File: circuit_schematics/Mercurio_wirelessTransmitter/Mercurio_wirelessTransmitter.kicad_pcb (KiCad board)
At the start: 2 copper layers, 120.6 x 52.1 mm, 61 parts, among them J1 USB_MICRO_B, J2 SIM_CARD_SLOT, J3 MAIN_ANTENNA, J4 SENSOR_IN, J5 ICSP, Q1 CSD16301Q2, Q2 CSD16301Q2, Q3 S8050, Q4 S8050, U1 ATmega8U2-MU, U2 SIM7600E-H, U3 ADS1115IDGS, U4 BQ29707DSET, U5 MT3608, Y1 16MHz

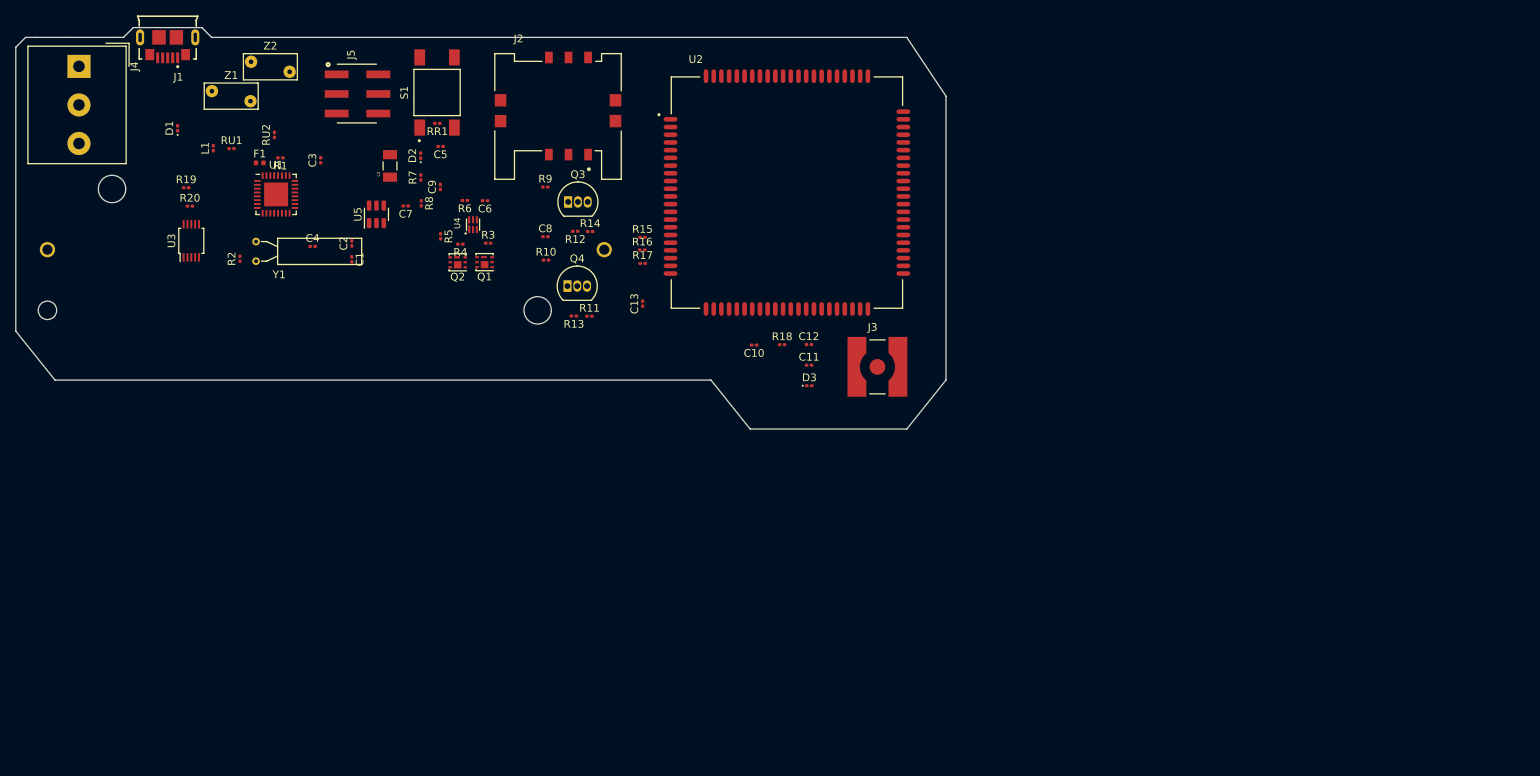
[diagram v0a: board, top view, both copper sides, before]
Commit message: Finalizada a PCB 2D e 3D, documentado esquematico e vistas de PCB 2D e 3D
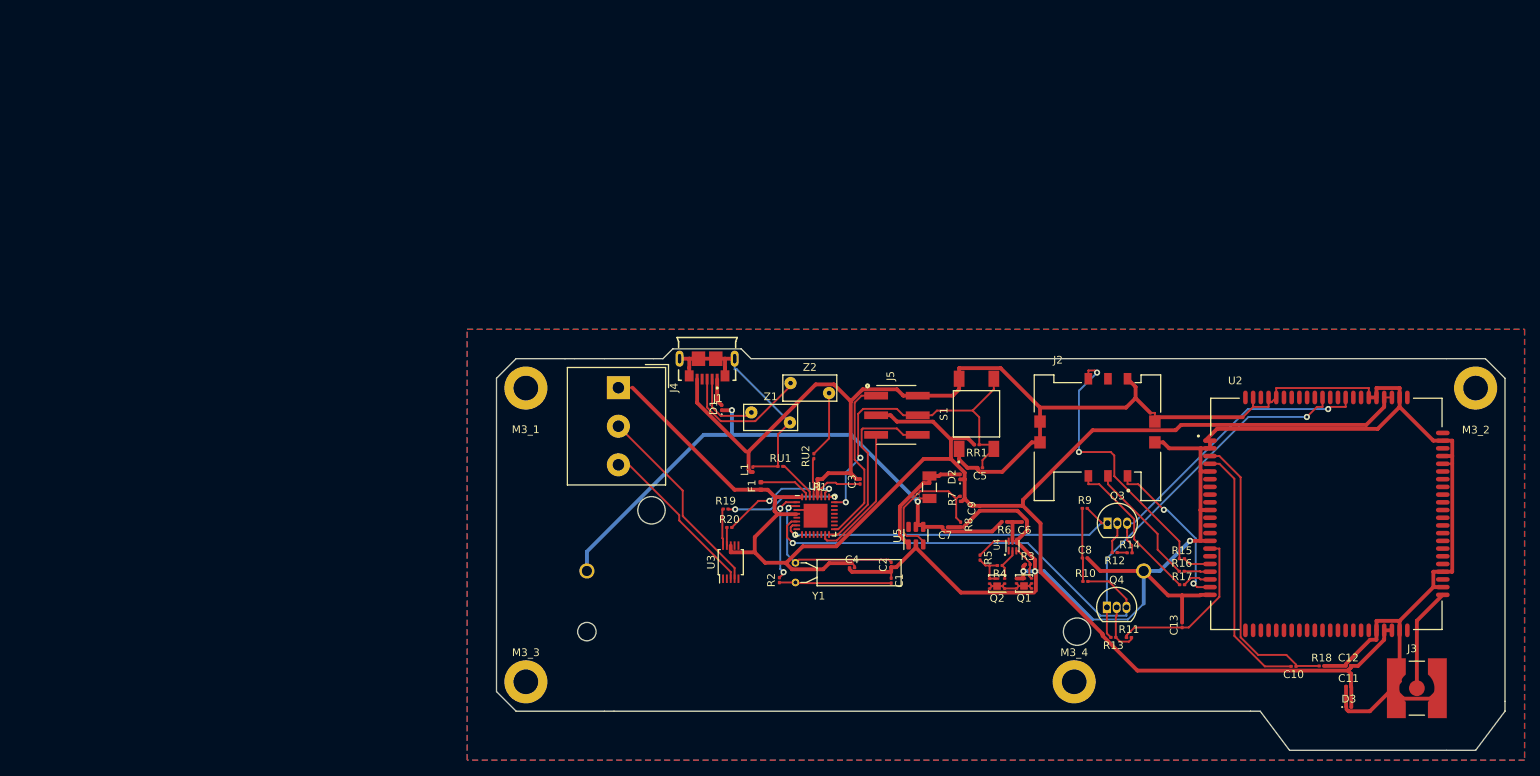
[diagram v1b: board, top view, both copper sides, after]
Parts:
- added M3_1: MountingHole_3.2mm_M3_DIN965_Pad, MountingHole:MountingHole_3.2mm_M3_DIN965_Pad, F.Cu at (85.2, 76.0)
- added M3_2: MountingHole_3.2mm_M3_DIN965_Pad, MountingHole:MountingHole_3.2mm_M3_DIN965_Pad, F.Cu at (208.4, 76.0)
- added M3_3: MountingHole_3.2mm_M3_DIN965_Pad, MountingHole:MountingHole_3.2mm_M3_DIN965_Pad, F.Cu at (85.2, 114.1)
- added M3_4: MountingHole_3.2mm_M3_DIN965_Pad, MountingHole:MountingHole_3.2mm_M3_DIN965_Pad, F.Cu at (156.3, 114.1)
- moved RU1 82.3 mm to (118.2, 86.1)
- moved Q2 81.4 mm to (146.3, 101.3)
- moved R3 81.4 mm to (150.3, 98.8)
- moved R20 81.4 mm to (111.6, 94.0)
- moved C5 81.4 mm to (144.1, 86.3)
- moved R1 81.4 mm to (123.3, 87.8)
- moved U3 81.4 mm to (111.8, 98.5)
- moved D3 81.4 mm to (192.0, 117.3)
- moved C4 81.4 mm to (127.5, 99.3)
- moved C9 81.4 mm to (144.1, 91.6)
- moved R6 81.4 mm to (147.3, 93.3)
- moved R19 81.4 mm to (111.1, 91.7)
- moved C8 81.4 mm to (157.7, 98.0)
- moved C10 81.4 mm to (184.8, 112.1)
- moved U4 81.4 mm to (148.3, 96.5)
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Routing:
- net GND: track 0.00 -> 403.1 mm, vias 0 -> 3
- net VBAT: track 0.00 -> 241.8 mm
- net Net-(BATTERY1-PadP): track 0.00 -> 76.9 mm, vias 0 -> 2
- net RXA: track 0.00 -> 59.3 mm, vias 0 -> 1
- net Net-(Q4-Pad1): track 0.00 -> 47.8 mm, vias 0 -> 1
- net TXA: track 0.00 -> 46.8 mm, vias 0 -> 1
- net Net-(C5-Pad1): track 0.00 -> 44.8 mm, vias 0 -> 2
- net Net-(Q3-Pad3): track 0.00 -> 39.9 mm, vias 0 -> 1
- net Net-(C10-Pad1): track 0.00 -> 37.8 mm
- net SIM_DATA: track 0.00 -> 35.2 mm, vias 0 -> 2
- net Net-(C10-Pad2): track 0.00 -> 33.4 mm
- net Net-(L1-Pad2): track 0.00 -> 32.7 mm
- net Net-(J4-Pad2): track 0.00 -> 26.0 mm
- net Net-(J5-Pad4): track 0.00 -> 24.4 mm
- net Net-(J5-Pad1): track 0.00 -> 22.0 mm
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- added copper zone on B.Cu, net GND
- added copper zone on F.Cu, net GND
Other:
- board size 120.6 x 52.1 mm -> 130.8 x 52.1 mm
